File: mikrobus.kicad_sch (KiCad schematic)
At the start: 12 parts, among them CON1 MIKROBUS_HOST_CONN, U11 MCP9808

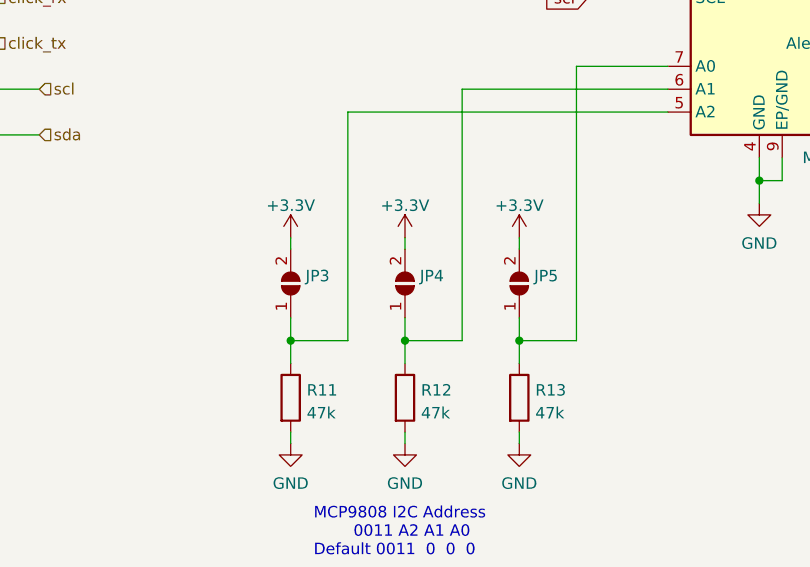
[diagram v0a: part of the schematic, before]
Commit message: Changed to KiCAD 7 and updated to final pinout.
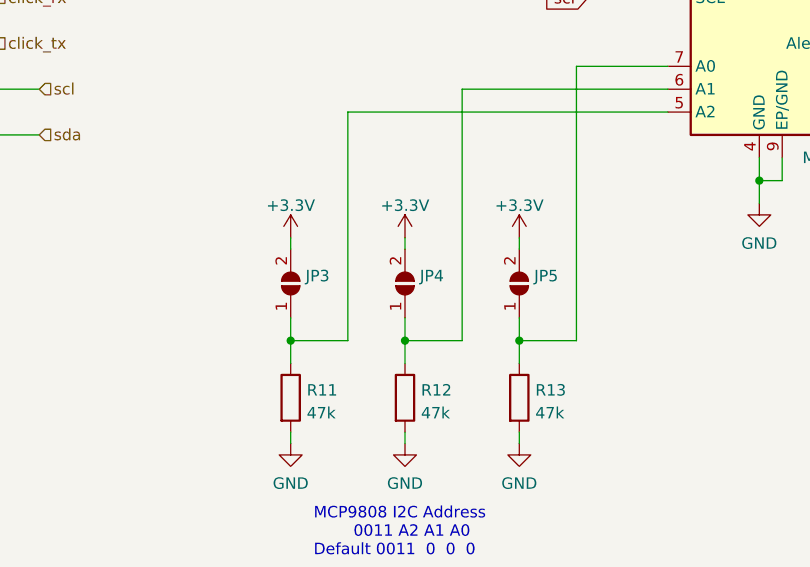
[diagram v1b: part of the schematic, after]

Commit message: updated footprints, added the barrel power connector and test points
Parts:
- CON1: footprint mikroBUS:MIKROBUS_HOST_CONN -> mikroBus:MIKROBUS_HOST_CONN
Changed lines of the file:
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@@
-    )
-  )
-  (symbol (lib_id "mikrobus:MIKROBUS_HOST_CONN") (at 62.23 109.22 0) (unit 1)
-    (in_bom yes) (on_board yes) (dnp no) (fields_autoplaced)
-    (property "Reference" "CON1" (at 76.2 64.8802 0)
-      (effects (font (size 1.27 1.27)))
-    )
-    (property "Value" "MIKROBUS_HOST_CONN" (at 76.2 67.4171 0)
-      (effects (font (size 1.27 1.27)))
-    )
-    (property "Footprint" "mikroBUS:MIKROBUS_HOST_CONN" (at 66.04 73.66 0)
-      (effects (font (size 1.27 1.27)) (justify left bottom) hide)
-    )
-    (property "Datasheet" "" (at 62.23 109.22 0)
-      (effects (font (size 1.27 1.27)) hide)
-    )
-    (pin "P1")
-    (pin "P10")
-    (pin "P11")
-    (pin "P12")
-    (pin "P13")
-    (pin "P14")
-    (pin "P15")
-    (pin "P16")
-    (pin "P2")
-    (pin "P3")
-    (pin "P4")
-    (pin "P5")
-    (pin "P6")
-    (pin "P7")
-    (pin "P8")
-    (pin "P9")
-    (instances
-      (project "OpenHW DevKit"
-        (path "/b0906e10-2fbc-4309-a8b4-6fc4cd1a5490/43d030b0-c46c-4448-bc9e-987f12c7559d"
-          (reference "CON1") (unit 1)
-        )
-      )
     )
   )
@@
         )
       )
+    )
+  )
+  (symbol (lib_id "mikrobus:MIKROBUS_HOST_CONN") (at 62.23 109.22 0) (unit 1)
+    (in_bom yes) (on_board yes) (dnp no) (fields_autoplaced)
+    (property "Reference" "CON1" (at 76.2 64.8802 0)
+      (effects (font (size 1.27 1.27)))
+    )
+    (property "Value" "MIKROBUS_HOST_CONN" (at 76.2 67.4171 0)
+      (effects (font (size 1.27 1.27)))
+    )
+    (property "Footprint" "mikroBus:MIKROBUS_HOST_CONN" (at 66.04 73.66 0)
+      (effects (font (size 1.27 1.27)) (justify left bottom) hide)
+    )
+    (property "Datasheet" "" (at 62.23 109.22 0)
+      (effects (font (size 1.27 1.27)) hide)
+    )
+    (pin "P1")
+    (pin "P10")
+    (pin "P11")
+    (pin "P12")
+    (pin "P13")
+    (pin "P14")
+    (pin "P15")
+    (pin "P16")
+    (pin "P2")
+    (pin "P3")
+    (pin "P4")
+    (pin "P5")
+    (pin "P6")
+    (pin "P7")
+    (pin "P8")
+    (pin "P9")
+    (instances
+      (project "OpenHW DevKit"
+        (path "/b0906e10-2fbc-4309-a8b4-6fc4cd1a5490/43d030b0-c46c-4448-bc9e-987f12c7559d"
+          (reference "CON1") (unit 1)
+        )
+        (path "/b0906e10-2fbc-4309-a8b4-6fc4cd1a5490/0f04658e-bc58-402e-baec-b0a803f67eac"
+          (reference "CON1") (unit 1)
+        )
+      )
